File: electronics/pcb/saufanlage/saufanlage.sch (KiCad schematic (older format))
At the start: 36 parts

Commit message: Backup commit
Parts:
- removed C? (x4): C, symbol Device:C
- removed D?: D_Schottky, symbol Device:D_Schottky
- removed J?: Conn_02x20_Odd_Even, symbol Connector_Generic:Conn_02x20_Odd_Even
- removed J?: Screw_Terminal_01x02, symbol Connector:Screw_Terminal_01x02
- removed J? (x4): Conn_01x03_Male, symbol Connector:Conn_01x03_Male
- removed J?: Conn_01x02_Female, symbol Connector:Conn_01x02_Female
- removed J?: Conn_01x05_Male, symbol Connector:Conn_01x05_Male
- removed L?: L, symbol Device:L
- removed R? (x6): R, symbol Device:R
- removed SW?: SW_Push, symbol Switch:SW_Push
- removed U?: BD9G341EFJ, Package_SO:HTSOP-8-1EP_3.9x4.9mm_P1.27mm_EP2.4x3.2mm_ThermalVias, symbol Regulator_Switching:BD9G341EFJ
- added J1, J10, J11, J12, J16, J17, J3, J4: Conn_01x08_Male, Connector_PinHeader_2.54mm:PinHeader_1x08_P2.54mm_Vertical, symbol Connector:Conn_01x08_Male
- added J13: Conn_02x03_Odd_Even, Connector_PinHeader_2.54mm:PinHeader_2x03_P2.54mm_Vertical, symbol Connector_Generic:Conn_02x03_Odd_Even
- added J14: Conn_02x18_Odd_Even, Connector_PinHeader_2.54mm:PinHeader_2x18_P2.54mm_Vertical, symbol Connector_Generic:Conn_02x18_Odd_Even
- added J15, J27: Conn_01x10_Male, Connector_PinHeader_2.54mm:PinHeader_1x10_P2.54mm_Vertical, symbol Connector:Conn_01x10_Male
- added J18: Conn_01x04, Connector_PinHeader_2.54mm:PinHeader_1x04_P2.54mm_Vertical, symbol Connector_Generic:Conn_01x04
- added J2: Screw_Terminal_01x02, Connector_Phoenix_MC:PhoenixContact_MCV_1,5_2-G-3.81_1x02_P3.81mm_Vertical, symbol Connector:Screw_Terminal_01x02
- added J23, J24, J29, J30, J31, J32: Conn_01x15_Male, Connector_PinHeader_2.54mm:PinHeader_1x15_P2.54mm_Vertical, symbol Connector:Conn_01x15_Male
- added J7, J9: Conn_01x20_Male, Connector_PinHeader_2.54mm:PinHeader_1x20_P2.54mm_Vertical, symbol Connector:Conn_01x20_Male
- added PS1, PS2: LM2596, saufanlage:LM2596, symbol saufanlage:LM2596
- J19: renamed from J?; footprint (none) -> Connector_PinHeader_2.54mm:PinHeader_1x06_P2.54mm_Vertical
- J20: renamed from J?; footprint (none) -> Connector_PinHeader_2.54mm:PinHeader_1x07_P2.54mm_Vertical
- J21, J25, J26, J28: renamed from J?; footprint (none) -> Connector_PinHeader_2.54mm:PinHeader_1x03_P2.54mm_Vertical
- J22: renamed from J?; footprint (none) -> Connector_PinHeader_2.54mm:PinHeader_1x10_P2.54mm_Vertical
- J5, J6: renamed from J?; footprint (none) -> Connector_PinHeader_2.54mm:PinHeader_2x08_P2.54mm_Vertical
- J8: renamed from J?; footprint (none) -> Connector_PinHeader_2.54mm:PinHeader_2x20_P2.54mm_Vertical
- XA1: renamed from XA?; footprint (none) -> Arduino:Arduino_Mega2560_Shield
- XA2, XA3, XA4: renamed from XA?; footprint (none) -> Arduino:Arduino_Nano_Socket
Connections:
- net labels added: +3.3V, +3V3, +5V, +8V, DT1, DT2, DT3, DT4, Fingerprint, Flowmeter1, Flowmeter2, Flowmeter3, Flowmeter4, MEGA_D20_SDA, MEGA_D21_SCL, MEGA_RX0, MEGA_RX1, MEGA_RX2, MEGA_RX3, MEGA_RX4, MEGA_TX0, MEGA_TX1, MEGA_TX2, MISO, MOSI, M_3V3, M_5V, M_A0, M_A1, M_A10, M_A11, M_A12, M_A13, M_A14, M_A15, M_A2, M_A3, M_A4, M_A5, M_A6, M_A7, M_A8, M_A9, M_AREF, M_D10, M_D11, M_D12, M_D13, M_D2, M_D22, M_D23, M_D24, M_D25, M_D26, M_D27, M_D28, M_D29, M_D3, M_D30, M_D31, M_D32, M_D33, M_D34, M_D35, M_D36, M_D37, M_D38, M_D39, M_D4, M_D46, M_D47, M_D48, M_D49, M_D5, M_D50, M_D51, M_D52, M_D53, M_D6, M_D7, M_D8, M_D9, M_IORF, M_MISO, M_MOSI, M_RST1, M_RST2, M_SCK, M_SPI_5V, N1_3V3, N1_5V, N1_A0, N1_A1, N1_A2, N1_A3, N1_A6, N1_A7, N1_AREF, N1_D0, N1_D1, N1_D10, N1_D11, N1_D12, N1_D13, N1_D2_INT0, N1_D3_INT1, N1_D4, N1_D5, N1_D6, N1_D7, N1_D8, N1_D9, N1_RST1, N1_RST2, N2_3V3, N2_5V, N2_A0, N2_A1, N2_A2, N2_A3, N2_A6, N2_A7, N2_AREF, N2_D0, N2_D1, N2_D10, N2_D11, N2_D12, N2_D13, N2_D2_INT0, N2_D3_INT1, N2_D4, N2_D5, N2_D6, N2_D7, N2_D8, N2_D9, N2_RST1, N2_RST2, N3_3V3, N3_5V, N3_A0, N3_A1, N3_A2, N3_A3, N3_A6, N3_A7, N3_AREF, N3_D0, N3_D1, N3_D10, N3_D11, N3_D12, N3_D13, N3_D2_INT0, N3_D3_INT1, N3_D4, N3_D5, N3_D6, N3_D7, N3_D8, N3_D9, N3_RST1, N3_RST2, RELAIS1, RELAIS2, RELAIS3, RELAIS4, RELAIS5, RELAIS6, RPI_GPIO10, RPI_GPIO11, RPI_GPIO12, RPI_GPIO13, RPI_GPIO14, RPI_GPIO15, RPI_GPIO16, RPI_GPIO17, RPI_GPIO18, RPI_GPIO19, RPI_GPIO20, RPI_GPIO21, RPI_GPIO22, RPI_GPIO23, RPI_GPIO24, RPI_GPIO25, RPI_GPIO26, RPI_GPIO27, RPI_GPIO4, RPI_GPIO5, RPI_GPIO6, RPI_GPIO7, RPI_GPIO8, RPI_GPIO9, RPI_IDSC, RPI_IDSD, RST, SCK, SCK1, SCK2, SCK3, SCK4, UART_RX, UART_TX
- wire segments 249 -> 594
- no-connect marks 0 -> 1
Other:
- note added: "Fingerprint"
- note added: "Flowmeter"
- note added: "LED Matrix Connection"
- note added: "Mega Breakout"
- note added: "NFC"
- note added: "Nano #1 Breakout"
- note added: "Nano #2 Breakout"
- note added: "Nano #3 Breakout"
- note added: "Power Input"
- note added: "RPi Breakout"
- note added: "Scale1"
- note added: "Scale2"
- note removed: "Buck Converter"
- note removed: "Flowmeter-connection"
- note removed: "Raspberry - reset"
- moved on the sheet: J19, J20, J21, J22, J25, J26, J28, J5, J6, J8, XA1, XA2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

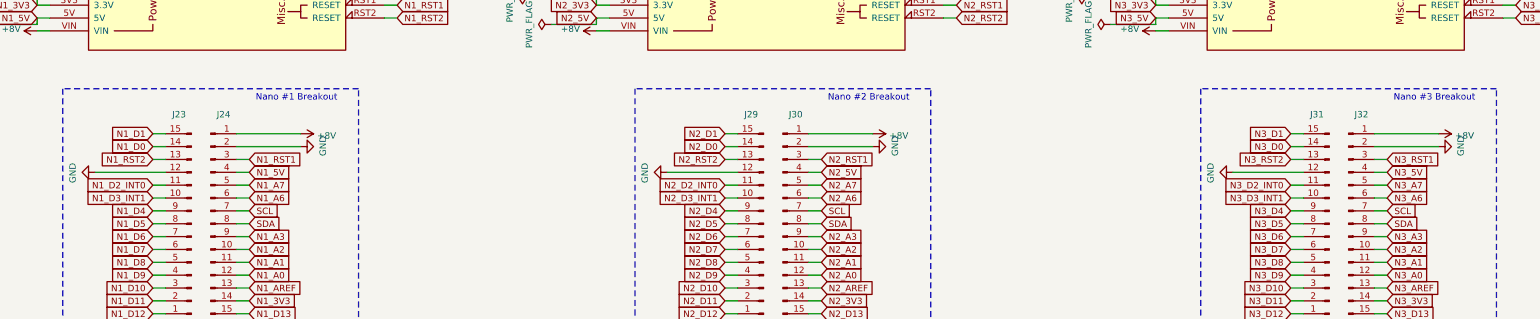
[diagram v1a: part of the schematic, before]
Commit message: More brainz updates
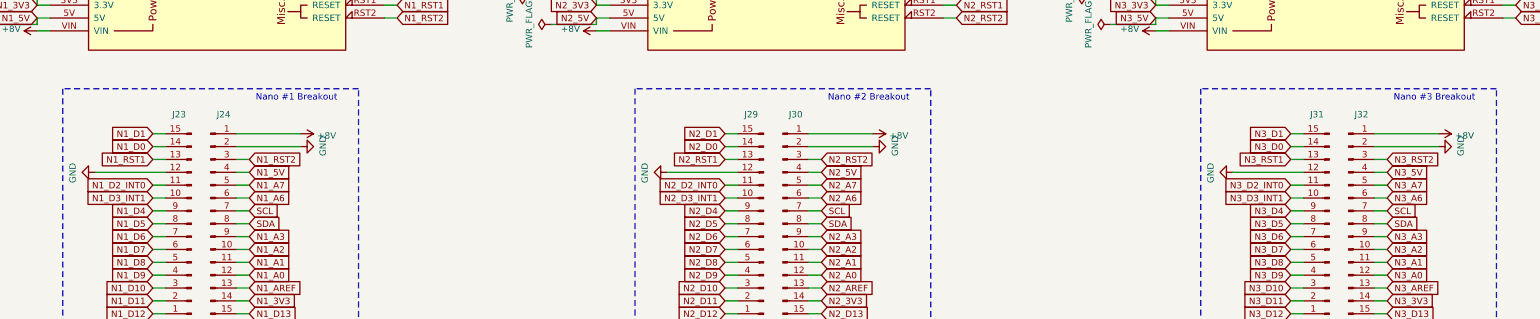
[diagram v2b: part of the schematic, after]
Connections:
- net N1_RST1: now also J23.13 (Pin_13); no longer J24.3 (Pin_3)
- net N1_RST2: now also J24.3 (Pin_3); no longer J23.13 (Pin_13)
- net N2_RST1: now also J29.13 (Pin_13); no longer J30.3 (Pin_3)
- net N2_RST2: now also J30.3 (Pin_3); no longer J29.13 (Pin_13)
- net N3_RST1: now also J31.13 (Pin_13); no longer J32.3 (Pin_3)
- net N3_RST2: now also J32.3 (Pin_3); no longer J31.13 (Pin_13)
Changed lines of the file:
@@
 	0    -1   -1   0
 $EndComp
-Text GLabel 12150 5300 2    50   Input ~ 0
-N1_RST1
 Text GLabel 12150 6200 2    50   Input ~ 0
 N1_A0
@@
 Text GLabel 12150 6300 2    50   Input ~ 0
 N1_AREF
-Text GLabel 11400 5300 0    50   Input ~ 0
-N1_RST2
 Wire Wire Line
 	11400 5200 11500 5200
@@
 	0    -1   -1   0
 $EndComp
-Text GLabel 16600 5300 2    50   Input ~ 0
-N2_RST1
 Text GLabel 16600 5700 2    50   Input ~ 0
 SCL
@@
 Text GLabel 16600 6300 2    50   Input ~ 0
 N2_AREF
-Text GLabel 15850 5300 0    50   Input ~ 0
-N2_RST2
 Wire Wire Line
 	15850 5200 15950 5200
@@
 	0    -1   -1   0
 $EndComp
-Text GLabel 21000 5300 2    50   Input ~ 0
-N3_RST1
 Text GLabel 21000 5500 2    50   Input ~ 0
 N3_A7
@@
 Text GLabel 21000 6300 2    50   Input ~ 0
 N3_AREF
-Text GLabel 20250 5300 0    50   Input ~ 0
-N3_RST2
 Wire Wire Line
 	20250 5200 20350 5200
@@
 Wire Wire Line
 	8150 8050 8200 8050
+Text GLabel 21000 5300 2    50   Input ~ 0
+N3_RST2
+Text GLabel 20250 5300 0    50   Input ~ 0
+N3_RST1
+Text GLabel 16600 5300 2    50   Input ~ 0
+N2_RST2
+Text GLabel 15850 5300 0    50   Input ~ 0
+N2_RST1
+Text GLabel 12150 5300 2    50   Input ~ 0
+N1_RST2
+Text GLabel 11400 5300 0    50   Input ~ 0
+N1_RST1
 $EndSCHEMATC
